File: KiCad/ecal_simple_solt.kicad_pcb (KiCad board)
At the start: 4 copper layers, 28 x 28 mm, 18 parts, among them J1 PORT1, J2 PORT2, J3 GPIO, U1 BGS14PN10, U2 BGS14PN10, U3 BGS12PN10, U4 BGS12PN10

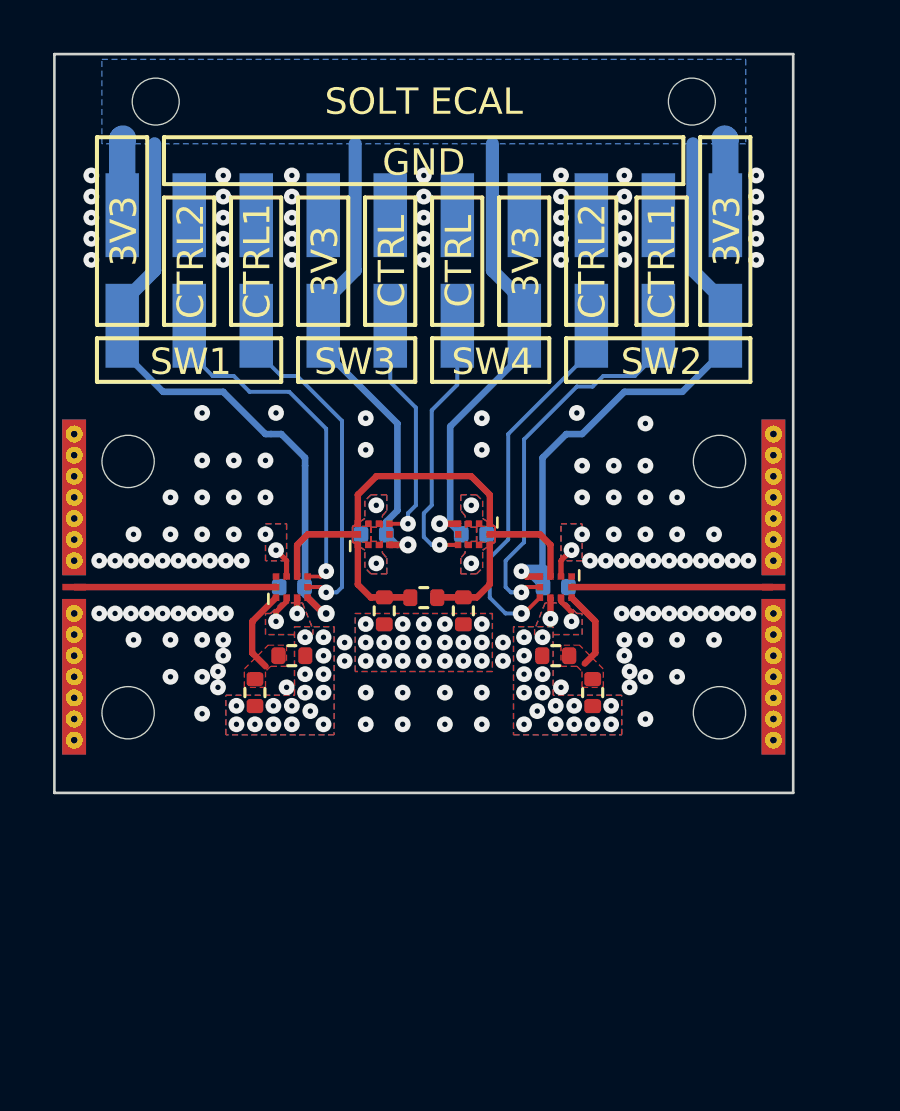
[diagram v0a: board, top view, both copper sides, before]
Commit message: New revision
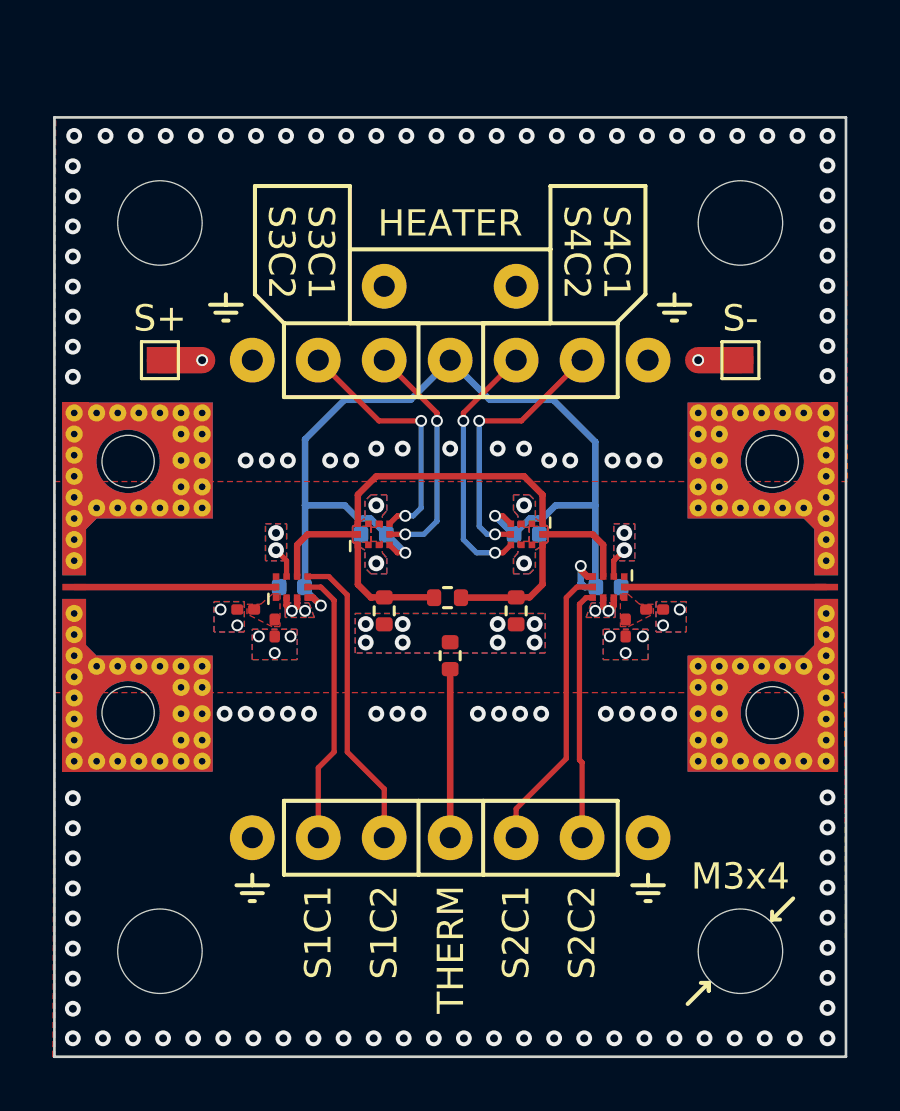
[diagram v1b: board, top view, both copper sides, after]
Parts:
- added H1: MountingHole, MountingHole:MountingHole_3.2mm_M3_ISO7380, F.Cu at (81.0, 60.4)
- added H2: MountingHole, MountingHole:MountingHole_3.2mm_M3_ISO7380, F.Cu at (103.0, 60.4)
- added H3: MountingHole, MountingHole:MountingHole_3.2mm_M3_ISO7380, F.Cu at (103.0, 88.0)
- added H4: MountingHole, MountingHole:MountingHole_3.2mm_M3_ISO7380, F.Cu at (81.0, 88.0)
- added J10: S4C1, Infineon:CPG-01-TH-B, B.Cu at (97.0, 65.6)
- added J11: S4C2, Infineon:CPG-01-TH-B, B.Cu at (94.5, 65.6)
- added J12: GND, Infineon:CPG-01-TH-B, B.Cu at (84.5, 83.7)
- added J13: GND, Infineon:CPG-01-TH-B, B.Cu at (99.5, 83.7)
- added J14: GND, Infineon:CPG-01-TH-B, B.Cu at (99.5, 65.6)
- added J15: 3V3, Infineon:CPG-01-TH-B, B.Cu at (92.0, 65.6)
- added J16: GND, Infineon:CPG-01-TH-B, B.Cu at (84.5, 65.6)
- added J17: HEAT, Infineon:CPG-01-TH-B, B.Cu at (94.5, 62.8)
- added J18: HEAT, Infineon:CPG-01-TH-B, B.Cu at (89.5, 62.8)
- added J4: S1C1, Infineon:CPG-01-TH-B, B.Cu at (87.0, 83.7)
- added J5: S1C2, Infineon:CPG-01-TH-B, B.Cu at (89.5, 83.7)
- added J6: S2C1, Infineon:CPG-01-TH-B, B.Cu at (94.5, 83.7)
- added J7: S2C2, Infineon:CPG-01-TH-B, B.Cu at (97.0, 83.7)
- added J8: S3C1, Infineon:CPG-01-TH-B, B.Cu at (89.5, 65.6)
- added J9: S3C2, Infineon:CPG-01-TH-B, B.Cu at (87.0, 65.6)
- added TH1: 10k, Resistor_SMD:R_0402_1005Metric, F.Cu at (92.0, 76.8)
- added TP1: TestPoint, TestPoint:TestPoint_Pad_1.0x1.0mm, F.Cu at (81.0, 65.6)
- added TP2: TestPoint, TestPoint:TestPoint_Pad_1.0x1.0mm, F.Cu at (103.0, 65.6)
- C1, C2, C3, C4: value C -> 100n
- J1, J2: footprint Infineon:1092-03A-6 -> Infineon:32K243-40ML5
- J3: value GPIO -> THERM; footprint Infineon:PinHeader_2x10_P2.54mm_Horizontal_SMD -> Infineon:CPG-01-TH-B
- R11, R12, R21, R22: footprint Resistor_SMD:R_0402_1005Metric -> Resistor_SMD:R_0201_0603Metric
- U3, U4: value BGS12PN10 -> BGS14PN10
- moved J3 21.5 mm to (92.0, 83.7)
- moved R21 3.93 mm to (99.8, 75.0), turned to 0 degrees
- moved R22 2.85 mm to (98.7, 75.8), turned to -90 degrees
- moved R11 2.56 mm to (85.3, 75.8)
- moved R12 2.47 mm to (84.2, 75.0), turned to 180 degrees
- moved C2 2.00 mm to (98.0, 74.2)
- moved C4 2.00 mm to (94.9, 72.2)
- moved J2 2.00 mm to (107.0, 74.2)
- moved R102 2.00 mm to (94.5, 75.1)
- moved U2 2.00 mm to (98.0, 74.2)
- moved U4 2.00 mm to (94.9, 72.2)
- moved R103 0.90 mm to (91.9, 74.6)
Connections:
- J3 pad 1: +3V3 -> /THERM
- U3 pad 3: GND -> unconnected-(U3-RF2-Pad3)
- U3 pad 5: unconnected-(U3-CTRL1-Pad5) -> SW3_CTRL1
- U3 pad 6: SW3_CTRL -> SW3_CTRL2
- U4 pad 3: GND -> unconnected-(U4-RF2-Pad3)
- U4 pad 5: unconnected-(U4-CTRL1-Pad5) -> SW4_CTRL1
- U4 pad 6: SW4_CTRL -> SW4_CTRL2
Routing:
- net /HEAT: track 0.00 -> 870.0 mm, vias 0 -> 2
- net +3V3: track 93.1 -> 38.9 mm
- net SW4_CTRL1: track 0.00 -> 10.2 mm, vias 0 -> 2
- net SW4_CTRL: track 9.96 -> 0.00 mm, vias 1 -> 0
- net SW4_CTRL2: track 0.00 -> 9.76 mm, vias 0 -> 2
- net SW3_CTRL2: track 0.00 -> 9.60 mm, vias 0 -> 2
- net SW3_CTRL1: track 0.00 -> 8.94 mm, vias 0 -> 2
- net SW3_CTRL: track 8.73 -> 0.00 mm, vias 1 -> 0
- net /THERM: track 0.00 -> 6.39 mm
- net SW2_CTRL2: track 14.3 -> 9.49 mm, vias 1 -> 0
- net SW2_CTRL1: track 14.8 -> 11.1 mm, vias 1 -> 0
- net SW1_Load: track 3.18 -> 0.00 mm
- net SW2_Load: track 3.04 -> 0.00 mm
- net SW1_CTRL1: track 13.1 -> 10.5 mm, vias 1 -> 0
- net SW1_CTRL2: track 13.6 -> 11.6 mm, vias 1 -> 0
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- removed copper zone on B.Cu, net +3V3
- removed copper zone on In2.Cu, net GND
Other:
- board size 28 x 28 mm -> 30 x 35.6 mm
- board text added: "HEATER"
- board text added: "M3x4"
- board text added: "S+"
- board text added: "S-"
- board text added: "S3C1"
- board text added: "S3C2"
- board text added: "S4C1"
- board text added: "S4C2"
- board text removed: "3V3"
- board text removed: "CTRL"
- board text removed: "CTRL1"
- board text removed: "CTRL2"
- board text removed: "GND"
- board text removed: "SOLT ECAL"
- board text removed: "SW1"
- board text removed: "SW2"
- board text removed: "SW3"
- board text removed: "SW4"
